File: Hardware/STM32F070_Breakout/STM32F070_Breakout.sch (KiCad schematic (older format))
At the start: 34 parts, among them J1 USB_B_Micro, J2 Conn_01x15, J3 Conn_01x15, J4 Conn_01x05, SW1 SW_Push, SW2 SW_Push, U1 AP2112K-3.3, U2 STM32F070CBT6, Y1 32.768kHZ, Y2 16MHz

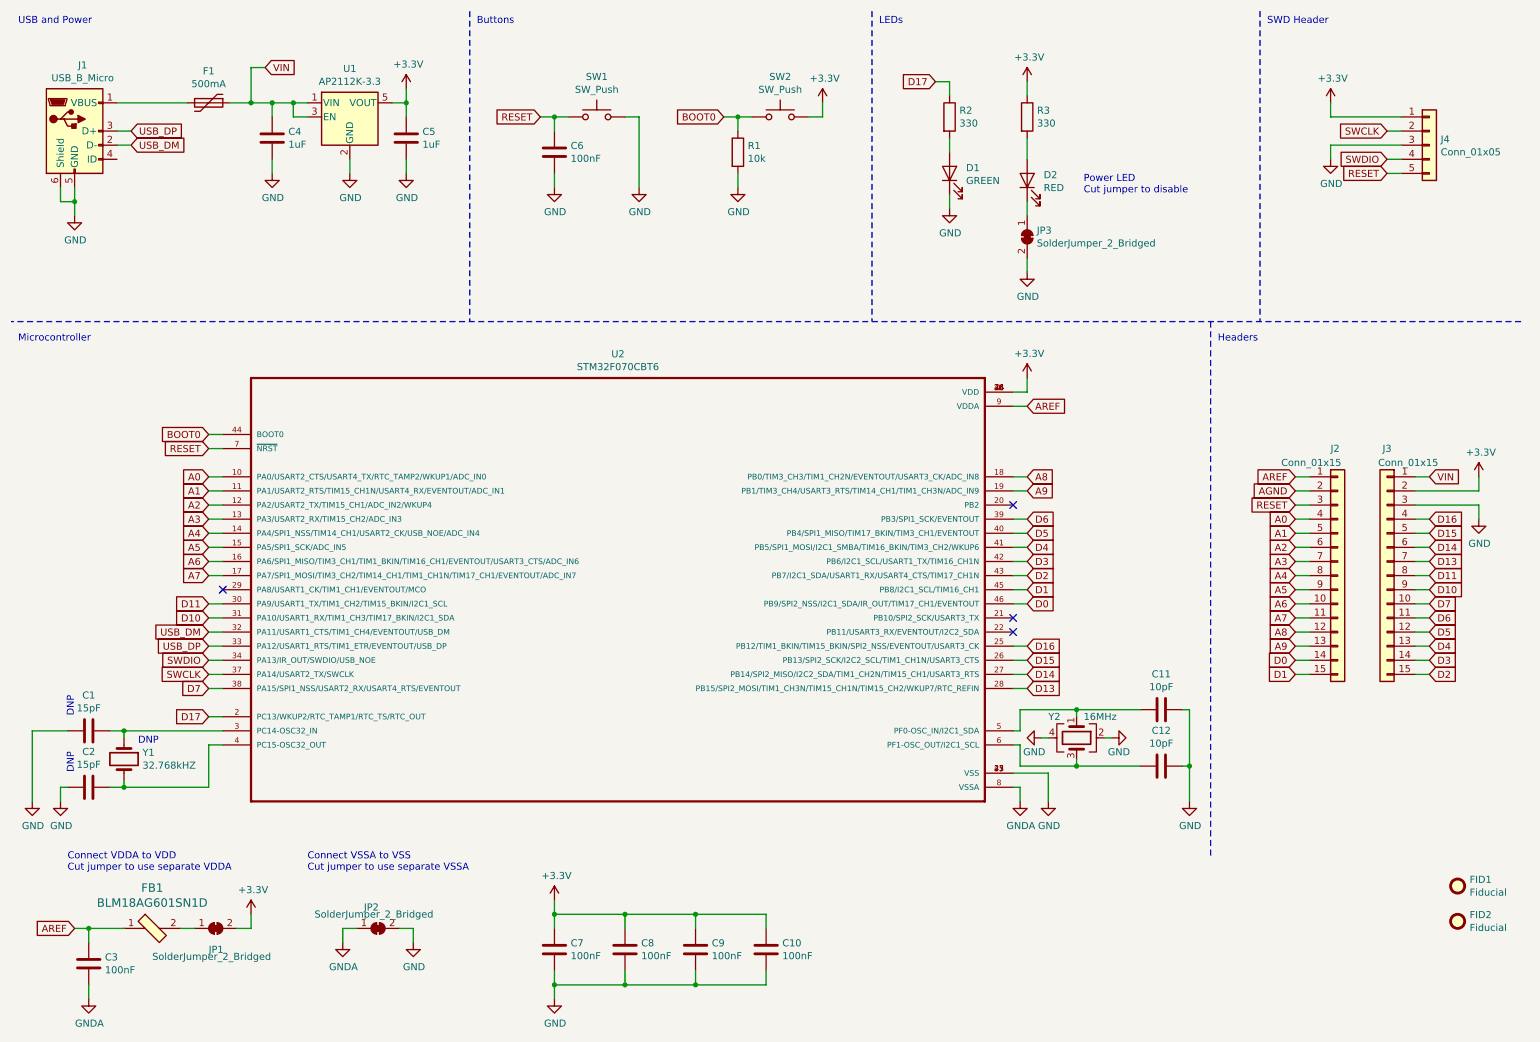
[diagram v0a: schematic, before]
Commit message: Components placed
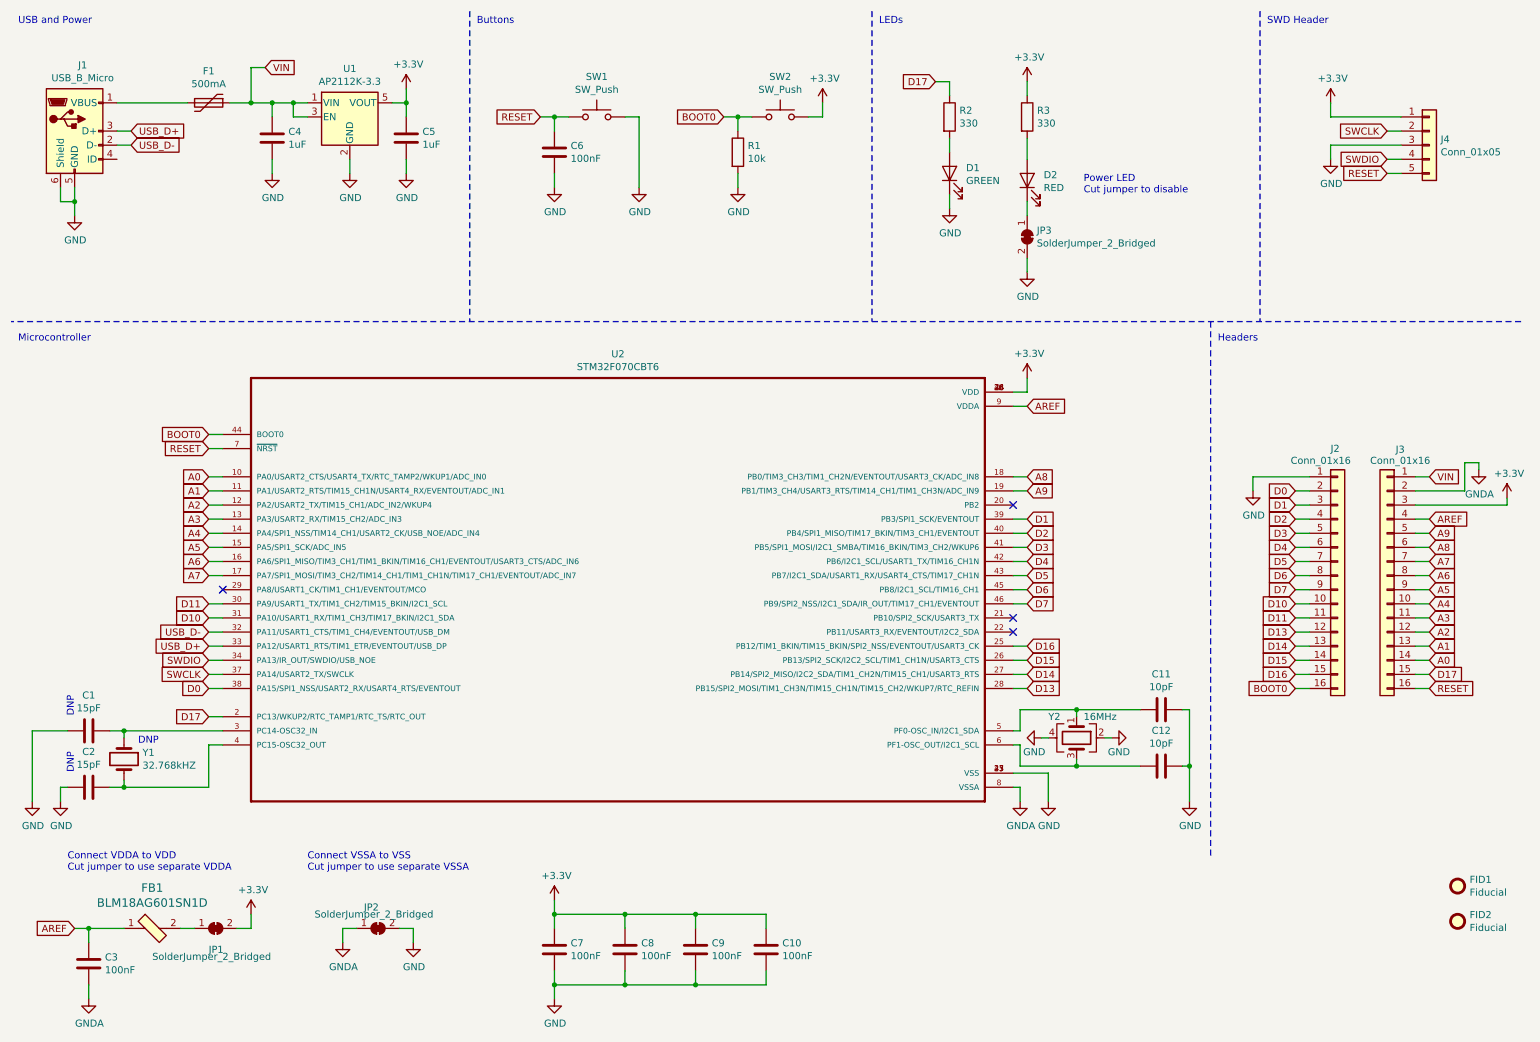
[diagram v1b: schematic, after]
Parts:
- removed J2, J3: Conn_01x15, Connector_PinHeader_2.54mm:PinHeader_1x15_P2.54mm_Vertical, symbol Connector_Generic:Conn_01x15
- added J2, J3: Conn_01x16, Connector_PinHeader_2.54mm:PinHeader_1x16_P2.54mm_Vertical, symbol Connector_Generic:Conn_01x16
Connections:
- net +3V3: now also J3.3 (Pin_3)
- net A0: now also J3.14 (Pin_14)
- net A1: now also J3.13 (Pin_13)
- net A2: now also J3.12 (Pin_12)
- net A3: now also J3.11 (Pin_11)
- net A4: now also J3.10 (Pin_10)
- net A5: now also J3.9 (Pin_9)
- net A6: now also J3.8 (Pin_8)
- net A7: now also J3.7 (Pin_7)
- net A8: now also J3.6 (Pin_6)
- net A9: now also J3.5 (Pin_5)
- net AREF: now also J3.4 (Pin_4)
- net BOOT0: now also J2.16 (Pin_16)
- net D0: now also U2.38 (PA15/SPI1_NSS/USART2_RX/USART4_RTS/EVENTOUT), J2.2 (Pin_2); no longer U2.46 (PB9/SPI2_NSS/I2C1_SDA/IR_OUT/TIM17_CH1/EVENTOUT)
- net D1: now also U2.39 (PB3/SPI1_SCK/EVENTOUT), J2.3 (Pin_3); no longer U2.45 (PB8/I2C1_SCL/TIM16_CH1)
- net D10: now also J2.10 (Pin_10)
- net D11: now also J2.11 (Pin_11)
- net D13: now also J2.12 (Pin_12)
- net D14: now also J2.13 (Pin_13)
- net D15: now also J2.14 (Pin_14)
- net D16: now also J2.15 (Pin_15)
- net D17: now also J3.15 (Pin_15)
- net D2: now also U2.40 (PB4/SPI1_MISO/TIM17_BKIN/TIM3_CH1/EVENTOUT), J2.4 (Pin_4); no longer U2.43 (PB7/I2C1_SDA/USART1_RX/USART4_CTS/TIM17_CH1N)
- net D3: now also U2.41 (PB5/SPI1_MOSI/I2C1_SMBA/TIM16_BKIN/TIM3_CH2/WKUP6), J2.5 (Pin_5); no longer U2.42 (PB6/I2C1_SCL/USART1_TX/TIM16_CH1N)
- net D4: now also U2.42 (PB6/I2C1_SCL/USART1_TX/TIM16_CH1N), J2.6 (Pin_6); no longer U2.41 (PB5/SPI1_MOSI/I2C1_SMBA/TIM16_BKIN/TIM3_CH2/WKUP6)
- net D5: now also U2.43 (PB7/I2C1_SDA/USART1_RX/USART4_CTS/TIM17_CH1N), J2.7 (Pin_7); no longer U2.40 (PB4/SPI1_MISO/TIM17_BKIN/TIM3_CH1/EVENTOUT)
- net D6: now also U2.45 (PB8/I2C1_SCL/TIM16_CH1), J2.8 (Pin_8); no longer U2.39 (PB3/SPI1_SCK/EVENTOUT)
- net D7: now also U2.46 (PB9/SPI2_NSS/I2C1_SDA/IR_OUT/TIM17_CH1/EVENTOUT), J2.9 (Pin_9); no longer U2.38 (PA15/SPI1_NSS/USART2_RX/USART4_RTS/EVENTOUT)
- net GND: now also J2.1 (Pin_1)
- net GNDA: now also J3.2 (Pin_2)
- net RESET: now also J3.16 (Pin_16)
- net VIN: now also J3.1 (Pin_1)
- net USB_DM renamed USB_D-
- net USB_DP renamed USB_D+
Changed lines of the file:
@@
 	1250 1450 1350 1450
 Text GLabel 1350 1350 2    50   Input ~ 0
-USB_DP
+USB_D+
 Text GLabel 1350 1450 2    50   Input ~ 0
-USB_DM
+USB_D-
 Wire Wire Line
 	1250 1150 1750 1150
@@
 Text Notes 550  600  0    50   ~ 0
 USB and Power
-$Comp
-L Connector_Generic:Conn_01x15 J2
-U 1 1 5CF20066
-P 9900 4500
-F 0 "J2" H 9850 5400 50  0000 L CNN
-F 1 "Conn_01x15" H 9500 5300 50  0000 L CNN
-F 2 "Connector_PinHeader_2.54mm:PinHeader_1x15_P2.54mm_Vertical" H 9900 4500 50  0001 C CNN
-F 3 "~" H 9900 4500 50  0001 C CNN
-	1    9900 4500
-	1    0    0    -1
-$EndComp
-$Comp
-L Connector_Generic:Conn_01x15 J3
-U 1 1 5CF226AE
-P 10250 4500
-F 0 "J3" H 10250 5400 50  0000 C CNN
-F 1 "Conn_01x15" H 10100 5300 50  0000 C CNN
-F 2 "Connector_PinHeader_2.54mm:PinHeader_1x15_P2.54mm_Vertical" H 10250 4500 50  0001 C CNN
-F 3 "~" H 10250 4500 50  0001 C CNN
-	1    10250 4500
-	-1   0    0    -1
-$EndComp
-Wire Wire Line
-	9700 3800 9600 3800
 Wire Wire Line
 	9700 3900 9600 3900
@@
 Wire Wire Line
 	9700 5200 9600 5200
-Text GLabel 9600 3800 0    50   Input ~ 0
-AREF
-Text GLabel 9600 3900 0    50   Input ~ 0
-AGND
-Text GLabel 9600 4000 0    50   Input ~ 0
-RESET
-Text GLabel 9600 4100 0    50   Input ~ 0
+Wire Wire Line
+	10450 5200 10550 5200
+Wire Wire Line
+	10450 5100 10550 5100
+Wire Wire Line
+	10450 5000 10550 5000
+Wire Wire Line
+	10450 4900 10550 4900
+Wire Wire Line
+	10450 4800 10550 4800
+Wire Wire Line
+	10450 4700 10550 4700
+Wire Wire Line
+	10450 4600 10550 4600
+Wire Wire Line
+	10450 4500 10550 4500
+Wire Wire Line
+	10450 4400 10550 4400
+Wire Wire Line
+	10450 4300 10550 4300
+Wire Wire Line
+	10450 3800 10550 3800
+Text GLabel 10550 5100 2    50   Input ~ 0
 A0
-Text GLabel 9600 4200 0    50   Input ~ 0
+Text GLabel 10550 5000 2    50   Input ~ 0
 A1
-Text GLabel 9600 4300 0    50   Input ~ 0
+Text GLabel 10550 4900 2    50   Input ~ 0
 A2
-Text GLabel 9600 4400 0    50   Input ~ 0
+Text GLabel 10550 4800 2    50   Input ~ 0
 A3
-Text GLabel 9600 4500 0    50   Input ~ 0
-A4
-Text GLabel 9600 4600 0    50   Input ~ 0
+Text GLabel 10550 4600 2    50   Input ~ 0
 A5
-Text GLabel 9600 4700 0    50   Input ~ 0
+Text GLabel 10550 4500 2    50   Input ~ 0
 A6
-Text GLabel 9600 4800 0    50   Input ~ 0
+Text GLabel 10550 4400 2    50   Input ~ 0
 A7
-Text GLabel 9600 4900 0    50   Input ~ 0
+Text GLabel 10550 4300 2    50   Input ~ 0
 A8
-Text GLabel 9600 5000 0    50   Input ~ 0
+Text GLabel 10550 4200 2    50   Input ~ 0
 A9
-Text GLabel 9600 5100 0    50   Input ~ 0
-D0
-Text GLabel 9600 5200 0    50   Input ~ 0
-D1
-Wire Wire Line
-	10450 5200 10550 5200
-Wire Wire Line
-	10450 5100 10550 5100
-Wire Wire Line
-	10450 5000 10550 5000
-Wire Wire Line
-	10450 4900 10550 4900
-Wire Wire Line
-	10450 4800 10550 4800
-Wire Wire Line
-	10450 4700 10550 4700
-Wire Wire Line
-	10450 4600 10550 4600
-Wire Wire Line
-	10450 4500 10550 4500
-Wire Wire Line
-	10450 4400 10550 4400
-Wire Wire Line
-	10450 4300 10550 4300
-Wire Wire Line
-	10450 4200 10550 4200
-Wire Wire Line
-	10450 4100 10550 4100
-Wire Wire Line
-	10450 3800 10550 3800
-Text GLabel 10550 5200 2    50   Input ~ 0
-D2
-Text GLabel 10550 5100 2    50   Input ~ 0
-D3
-Text GLabel 10550 5000 2    50   Input ~ 0
-D4
-Text GLabel 10550 4900 2    50   Input ~ 0
-D5
-Text GLabel 10550 4800 2    50   Input ~ 0
-D6
-Text GLabel 10550 4700 2    50   Input ~ 0
-D7
-Text GLabel 10550 4600 2    50   Input ~ 0
-D10
-Text GLabel 10550 4500 2    50   Input ~ 0
-D11
-Text GLabel 10550 4400 2    50   Input ~ 0
-D13
-Text GLabel 10550 4300 2    50   Input ~ 0
-D14
-Text GLabel 10550 4200 2    50   Input ~ 0
-D15
-Text GLabel 10550 4100 2    50   Input ~ 0
-D16
 Text GLabel 10550 3800 2    50   Input ~ 0
 VIN
@@
 L power:+3.3V #PWR028
 U 1 1 5CF45684
-P 10900 3800
-F 0 "#PWR028" H 10900 3650 50  0001 C CNN
-F 1 "+3.3V" H 10915 3973 50  0000 C CNN
-F 2 "" H 10900 3800 50  0001 C CNN
-F 3 "" H 10900 3800 50  0001 C CNN
-	1    10900 3800
-	1    0    0    -1
-$EndComp
-$Comp
-L power:GND #PWR029
-U 1 1 5CF4627F
-P 10900 4100
-F 0 "#PWR029" H 10900 3850 50  0001 C CNN
-F 1 "GND" H 10905 3927 50  0000 C CNN
-F 2 "" H 10900 4100 50  0001 C CNN
-F 3 "" H 10900 4100 50  0001 C CNN
-	1    10900 4100
-	1    0    0    -1
-$EndComp
-Wire Wire Line
-	10900 3900 10900 3800
-Wire Wire Line
-	10450 3900 10900 3900
-Wire Wire Line
-	10900 4000 10900 4100
-Wire Wire Line
-	10450 4000 10900 4000
+P 11100 3950
+F 0 "#PWR028" H 11100 3800 50  0001 C CNN
+F 1 "+3.3V" H 11115 4123 50  0000 C CNN
+F 2 "" H 11100 3950 50  0001 C CNN
+F 3 "" H 11100 3950 50  0001 C CNN
+	1    11100 3950
+	1    0    0    -1
+$EndComp
 Text Notes 9050 2850 0    50   ~ 0
 Headers
@@
 D10
 Text GLabel 1900 4900 0    50   Input ~ 0
-USB_DM
+USB_D-
 Text GLabel 1900 5000 0    50   Input ~ 0
-USB_DP
+USB_D+
 Text GLabel 1900 5100 0    50   Input ~ 0
 SWDIO
@@
 SWCLK
 Text GLabel 1900 5300 0    50   Input ~ 0
-D7
+D0
 Text GLabel 1900 5500 0    50   Input ~ 0
 D17
@@
 NoConn ~ 7600 4000
 Text GLabel 7700 4100 2    50   Input ~ 0
+D1
+Text GLabel 7700 4200 2    50   Input ~ 0
+D2
+Text GLabel 7700 4300 2    50   Input ~ 0
+D3
+Text GLabel 7700 4400 2    50   Input ~ 0
+D4
+Text GLabel 7700 4500 2    50   Input ~ 0
+D5
+Text GLabel 7700 4600 2    50   Input ~ 0
 D6
-Text GLabel 7700 4200 2    50   Input ~ 0
-D5
-Text GLabel 7700 4300 2    50   Input ~ 0
-D4
-Text GLabel 7700 4400 2    50   Input ~ 0
-D3
-Text GLabel 7700 4500 2    50   Input ~ 0
-D2
-Text GLabel 7700 4600 2    50   Input ~ 0
-D1
 Text GLabel 7700 4700 2    50   Input ~ 0
-D0
+D7
 NoConn ~ 7600 4800
 NoConn ~ 7600 4900
@@
 Wire Wire Line
 	8850 5850 8850 6100
+Text GLabel 9600 3900 0    50   Input ~ 0
+D0
+Text GLabel 9600 4000 0    50   Input ~ 0
+D1
+Text GLabel 9600 4100 0    50   Input ~ 0
+D2
+Text GLabel 9600 4200 0    50   Input ~ 0
+D3
+Text GLabel 9600 4300 0    50   Input ~ 0
+D4
+Text GLabel 9600 4400 0    50   Input ~ 0
+D5
+Text GLabel 9600 4500 0    50   Input ~ 0
+D6
+Text GLabel 9600 4600 0    50   Input ~ 0
+D7
+Text GLabel 9600 4700 0    50   Input ~ 0
+D10
+Text GLabel 9600 4800 0    50   Input ~ 0
+D11
+Text GLabel 9600 4900 0    50   Input ~ 0
+D13
+Text GLabel 9600 5000 0    50   Input ~ 0
+D14
+Text GLabel 9600 5100 0    50   Input ~ 0
+D15
+Text GLabel 9600 5200 0    50   Input ~ 0
+D16
+$Comp
+L power:GNDA #PWR0103
+U 1 1 5D02AF3F
+P 10900 3750
+F 0 "#PWR0103" H 10900 3500 50  0001 C CNN
+F 1 "GNDA" H 10905 3577 50  0000 C CNN
+F 2 "" H 10900 3750 50  0001 C CNN
+F 3 "" H 10900 3750 50  0001 C CNN
+	1    10900 3750
+	1    0    0    -1
+$EndComp
+Wire Wire Line
+	10450 4100 10550 4100
+Text GLabel 10550 4100 2    50   Input ~ 0
+AREF
+Text GLabel 10550 4700 2    50   Input ~ 0
+A4
+$Comp
+L power:GND #PWR0104
+U 1 1 5D05FB59
+P 9300 3900
+F 0 "#PWR0104" H 9300 3650 50  0001 C CNN
+F 1 "GND" H 9305 3727 50  0000 C CNN
+F 2 "" H 9300 3900 50  0001 C CNN
+F 3 "" H 9300 3900 50  0001 C CNN
+	1    9300 3900
+	1    0    0    -1
+$EndComp
+Wire Wire Line
+	9300 3800 9300 3900
+Wire Wire Line
+	9300 3800 9700 3800
+$Comp
+L Connector_Generic:Conn_01x16 J2
+U 1 1 5D06D550
+P 9900 4500
+F 0 "J2" H 9850 5400 50  0000 L CNN
+F 1 "Conn_01x16" H 9567 5315 50  0000 L CNN
+F 2 "Connector_PinHeader_2.54mm:PinHeader_1x16_P2.54mm_Vertical" H 9900 4500 50  0001 C CNN
+F 3 "~" H 9900 4500 50  0001 C CNN
+	1    9900 4500
+	1    0    0    -1
+$EndComp
+$Comp
+L Connector_Generic:Conn_01x16 J3
+U 1 1 5D06E7A9
+P 10250 4500
+F 0 "J3" H 10157 5394 50  0000 C CNN
+F 1 "Conn_01x16" H 10157 5315 50  0000 C CNN
+F 2 "Connector_PinHeader_2.54mm:PinHeader_1x16_P2.54mm_Vertical" H 10250 4500 50  0001 C CNN
+F 3 "~" H 10250 4500 50  0001 C CNN
+	1    10250 4500
+	-1   0    0    -1
+$EndComp
+Wire Wire Line
+	10450 3900 10800 3900
+Wire Wire Line
+	10800 3900 10800 3700
+Wire Wire Line
+	10800 3700 10900 3700
+Wire Wire Line
+	10900 3700 10900 3750
+Wire Wire Line
+	11100 4000 11100 3950
+Wire Wire Line
+	10450 4000 11100 4000
+Wire Wire Line
+	10450 5300 10550 5300
+Wire Wire Line
+	9700 5300 9600 5300
+Text GLabel 10550 5200 2    50   Input ~ 0
+D17
+Text GLabel 10550 5300 2    50   Input ~ 0
+RESET
+Text GLabel 9600 5300 0    50   Input ~ 0
+BOOT0
+Wire Wire Line
+	10450 4200 10550 4200
 $EndSCHEMATC
